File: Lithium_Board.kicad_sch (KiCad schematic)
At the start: 66 parts, among them IC1 BQ25750RRVR, IC2 TPS70933DBVR, J1 XT30PW-M, J2 XT30PW-F, J3 XT30PW-M, J5 TSW-105-07-G-S, Q1 SIR870ADP-T1-GE3, Q2 SIR870ADP-T1-GE3, Q3 SIR870ADP-T1-GE3, Q4 SIR870ADP-T1-GE3, Q5 SIR870ADP-T1-GE3, Q6 SIR870ADP-T1-GE3, Q7 SIR870ADP-T1-GE3, Q8 SIR870ADP-T1-GE3

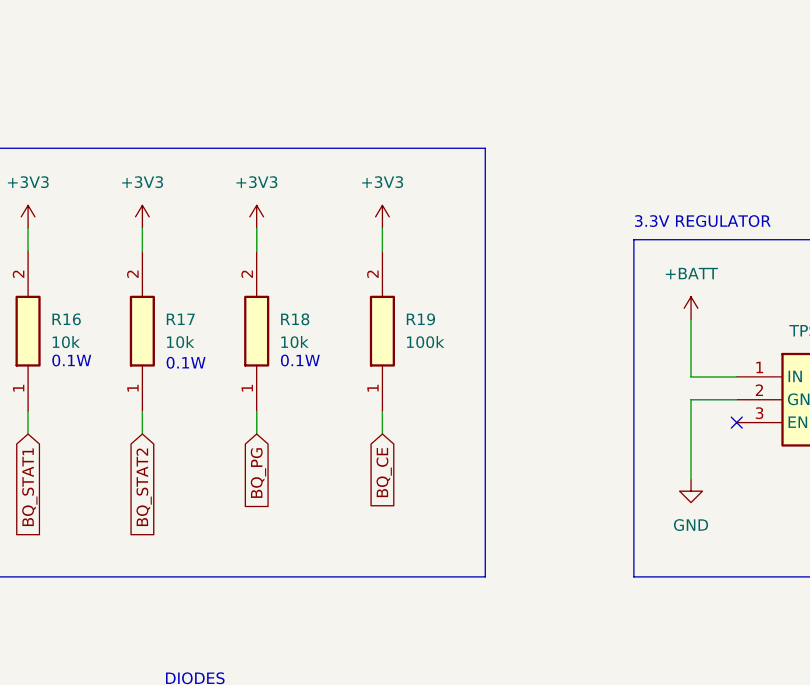
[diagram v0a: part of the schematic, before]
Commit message: Small Changes
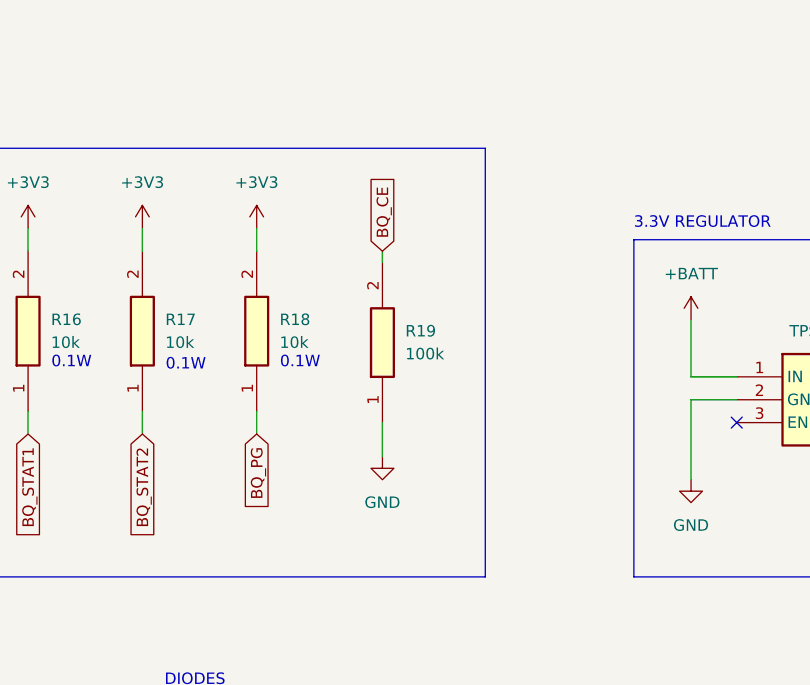
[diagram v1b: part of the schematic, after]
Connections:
- net +3V3: no longer R19.2
- net BQ_CE: now also R19.2; no longer R19.1
- net GND: now also R19.1
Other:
- moved on the sheet: R19
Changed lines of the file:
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@@
 	(wire
 		(pts
-			(xy 317.5 254) (xy 317.5 256.54)
-		)
-		(stroke
-			(width 0)
-			(type default)
-		)
-	)
-	(wire
-		(pts
 			(xy 83.82 86.36) (xy 83.82 83.82)
 		)
@@
 	(wire
 		(pts
+			(xy 317.5 275.59) (xy 317.5 279.4)
+		)
+		(stroke
+			(width 0)
+			(type default)
+		)
+	)
+	(wire
+		(pts
 			(xy 367.03 132.08) (xy 388.62 132.08)
 		)
@@
 	(wire
 		(pts
-			(xy 317.5 274.32) (xy 317.5 276.86)
-		)
-		(stroke
-			(width 0)
-			(type default)
-		)
-	)
-	(wire
-		(pts
 			(xy 290.83 274.32) (xy 290.83 276.86)
 		)
@@
 	(wire
 		(pts
+			(xy 317.5 256.54) (xy 317.5 257.81)
+		)
+		(stroke
+			(width 0)
+			(type default)
+		)
+	)
+	(wire
+		(pts
 			(xy 303.53 254) (xy 303.53 256.54)
 		)
@@
 	(global_label "BQ_CE"
 		(shape input)
-		(at 317.5 276.86 270)
+		(at 317.5 256.54 90)
 		(fields_autoplaced yes)
 		(effects
@@
 				(size 1.27 1.27)
 			)
-			(justify right)
+			(justify left)
 		)
 		(property "Intersheetrefs" "${INTERSHEET_REFS}"
-			(at 317.5 285.8323 90)
+			(at 317.5 247.5677 90)
 			(effects
 				(font
 					(size 1.27 1.27)
 				)
-				(justify right)
+				(justify left)
 				(hide yes)
 			)
@@
 	(symbol
 		(lib_id "RC0603FR-07100KL:RC0603FR-07100KL")
-		(at 317.5 274.32 90)
+		(at 317.5 275.59 90)
 		(unit 1)
 		(exclude_from_sim no)
@@
 		(fields_autoplaced yes)
 		(property "Reference" "R19"
-			(at 320.04 264.1599 90)
+			(at 320.04 265.4299 90)
 			(effects
 				(font
@@
 		)
 		(property "Value" "100k"
-			(at 320.04 266.6999 90)
+			(at 320.04 267.9699 90)
 			(effects
 				(font
@@
 		)
 		(property "Footprint" "RC0603FR-07100KL:RESC1608X55N"
-			(at 413.69 260.35 0)
+			(at 413.69 261.62 0)
 			(effects
 				(font
@@
 		)
 		(property "Datasheet" "https://www.yageo.com/upload/media/product/productsearch/datasheet/rchip/PYu-RC_Group_51_RoHS_L_12.pdf"
-			(at 513.69 260.35 0)
+			(at 513.69 261.62 0)
 			(effects
 				(font
@@
 		)
 		(property "Description" "100 kOhms +/-1% 0.1W, 1/10W Chip Resistor 0603 (1608 Metric) Moisture Resistant Thick Film"
-			(at 317.5 274.32 0)
+			(at 317.5 275.59 0)
 			(effects
 				(font
@@
 		)
 		(property "Height" "0.55"
-			(at 713.69 260.35 0)
+			(at 713.69 261.62 0)
 			(effects
 				(font
@@
 		)
 		(property "Mouser Part Number" "603-RC0603FR-07100KL"
-			(at 813.69 260.35 0)
+			(at 813.69 261.62 0)
 			(effects
 				(font
@@
 		)
 		(property "Mouser Price/Stock" "https://www.mouser.co.uk/ProductDetail/YAGEO/RC0603FR-07100KL?qs=e1ok2LiJcmaihem8Va5%2Fsw%3D%3D"
-			(at 913.69 260.35 0)
+			(at 913.69 261.62 0)
 			(effects
 				(font
@@
 		)
 		(property "Manufacturer_Name" "Yageo Group"
-			(at 1013.69 260.35 0)
+			(at 1013.69 261.62 0)
 			(effects
 				(font
@@
 		)
 		(property "Manufacturer_Part_Number" "RC0603FR-07100KL"
-			(at 1113.69 260.35 0)
+			(at 1113.69 261.62 0)
 			(effects
 				(font
@@
 	)
 	(symbol
+		(lib_id "power:GND")
+		(at 317.5 279.4 0)
+		(unit 1)
+		(exclude_from_sim no)
+		(in_bom yes)
+		(on_board yes)
+		(dnp no)
+		(fields_autoplaced yes)
+		(property "Reference" "#PWR019"
+			(at 317.5 285.75 0)
+			(effects
+				(font
+					(size 1.27 1.27)
+				)
+				(hide yes)
+			)
+		)
+		(property "Value" "GND"
+			(at 317.5 284.48 0)
+			(effects
+				(font
+					(size 1.27 1.27)
+				)
+			)
+		)
+		(property "Footprint" ""
+			(at 317.5 279.4 0)
+			(effects
+				(font
+					(size 1.27 1.27)
+				)
+				(hide yes)
+			)
+		)
+		(property "Datasheet" ""
+			(at 317.5 279.4 0)
+			(effects
+				(font
+					(size 1.27 1.27)
+				)
+				(hide yes)
+			)
+		)
+		(property "Description" "Power symbol creates a global label with name \"GND\" , ground"
+			(at 317.5 279.4 0)
+			(effects
+				(font
+					(size 1.27 1.27)
+				)
+				(hide yes)
+			)
+		)
+		(pin "1"
+		)
+		(instances
+			(project "Lithium_Board"
+				(path "/a208389b-7ee7-48d8-95f2-b3e129849547"
+					(reference "#PWR019")
+					(unit 1)
+				)
+			)
+		)
+	)
+	(symbol
 		(lib_id "RC0603FR-0710KL:RC0603FR-0710KL")
 		(at 265.43 274.32 90)
@@
 					(unit 1)
 				)
-			)
-		)
-	)
-	(symbol
-		(lib_id "power:+3V3")
-		(at 317.5 254 0)
-		(unit 1)
-		(exclude_from_sim no)
-		(in_bom yes)
-		(on_board yes)
-		(dnp no)
-		(fields_autoplaced yes)
-		(property "Reference" "#PWR019"
-			(at 317.5 257.81 0)
-			(effects
-				(font
-					(size 1.27 1.27)
-				)
-				(hide yes)
-			)
-		)
-		(property "Value" "+3V3"
-			(at 317.5 248.92 0)
-			(effects
-				(font
-					(size 1.27 1.27)
-				)
-			)
-		)
-		(property "Footprint" ""
-			(at 317.5 254 0)
-			(effects
-				(font
-					(size 1.27 1.27)
-				)
-				(hide yes)
-			)
-		)
-		(property "Datasheet" ""
-			(at 317.5 254 0)
-			(effects
-				(font
-					(size 1.27 1.27)
-				)
-				(hide yes)
-			)
-		)
-		(property "Description" "Power symbol creates a global label with name \"+3V3\""
-			(at 317.5 254 0)
-			(effects
-				(font
-					(size 1.27 1.27)
-				)
-				(hide yes)
-			)
-		)
-		(pin "1"
-		)
-		(instances
-			(project "Lithium_Board"
-				(path "/a208389b-7ee7-48d8-95f2-b3e129849547"
-					(reference "#PWR019")
-					(unit 1)
-				)

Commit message: TS fixed + Small Changes
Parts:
- added R32: 10k, RC0603FR-0710KL:RESC1608X55N, symbol RC0603FR-0710KL:RC0603FR-0710KL
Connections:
- net BQ_TS: now also R32.1
- net GND: now also R32.2
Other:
- moved on the sheet: D2, D5
